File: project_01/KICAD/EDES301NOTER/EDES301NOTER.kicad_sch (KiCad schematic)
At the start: 39 parts, among them Q1 S8050, Q2 BSS84, Q3 BSS84, Q4 BSS84, Q5 BSS138, Q7 BSS138, SW1 SW_Reed, U1 POCKETBEAGLE, U3 TPS613222ADBVR

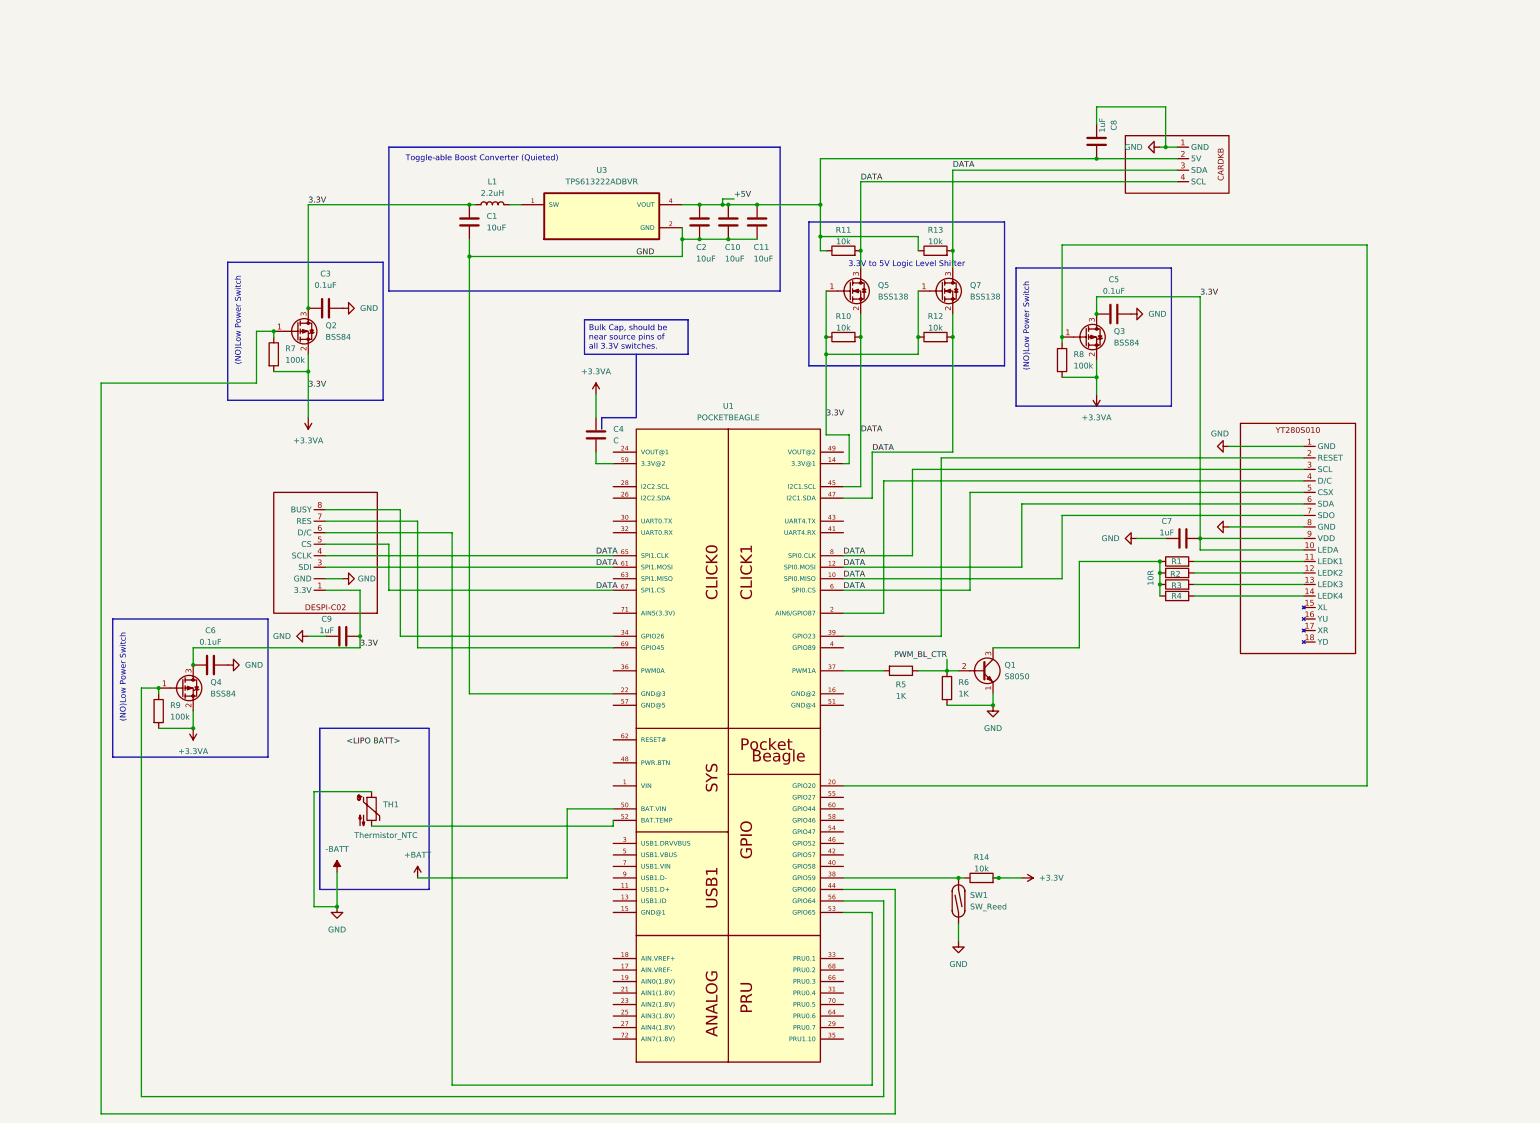
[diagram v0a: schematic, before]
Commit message: UpdateSchematicV1
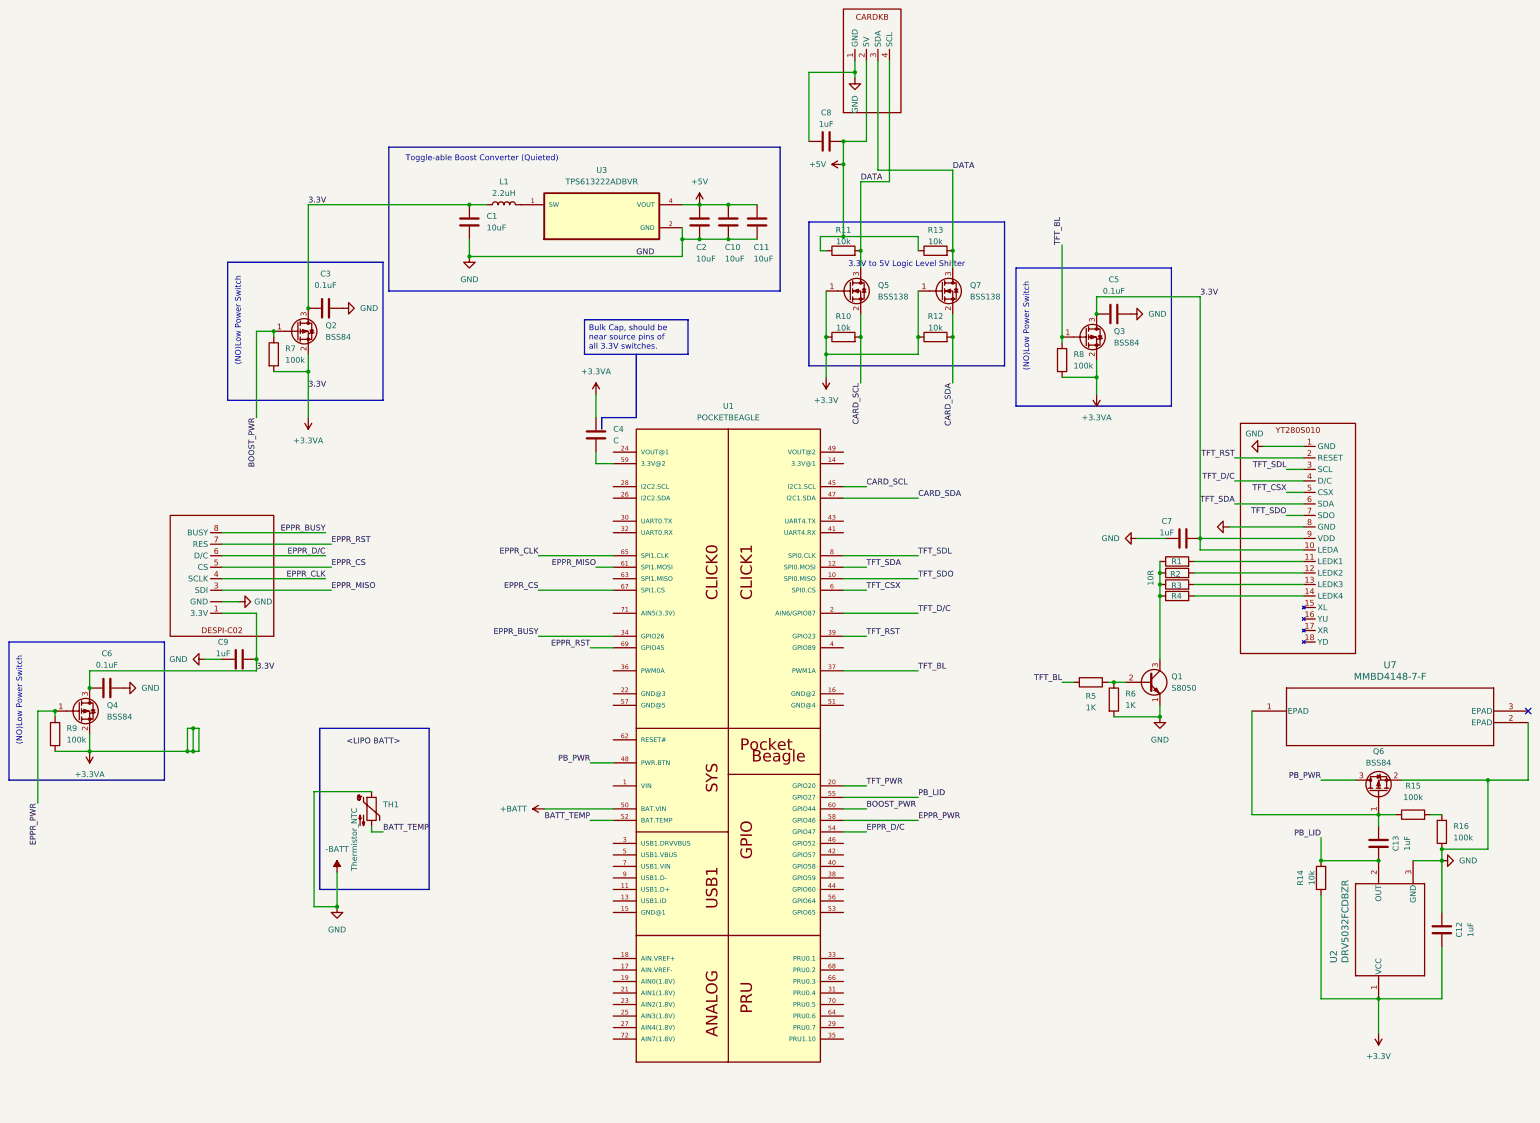
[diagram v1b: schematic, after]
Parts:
- removed SW1: SW_Reed, symbol Switch:SW_Reed
- added C12, C13: 1uF, Footprints:CAPC1608X90N, symbol Device:C
- added Q6: BSS84, Package_TO_SOT_SMD:SOT-23, symbol Transistor_FET:BSS84
- added R15, R16: 100k, Footprints:RESC1607X60N, symbol Device:R
- added U2: DRV5032FCDBZR, DBZ0003A-IPC_A, symbol DRV5032FCDBZR:DRV5032FCDBZR
- added U7: MMBD4148-7-F, SOT-23_DIO, symbol MMBD4148-7-F:MMBD4148-7-F
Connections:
- net +3.3V: now also Q5.1 (G), Q7.1 (G), R10.1, R12.1, R14.1, C12.1, U2.1 (VCC); no longer R14.2
- net +3.3VA: no longer Q5.1 (G), Q7.1 (G), R10.1, R12.1, U1.14 (3.3V@1)
- net -BATT: now also C12.2, Q6.2 (S), R16.1, U2.3 (GND), U7.2 (EPAD); no longer U1.22 (GND@3)
- net DATA: now also Q7.3 (D), R13.2, U4.3 (SDA); no longer Q5.2 (S), Q7.2 (S), R10.2, R12.2, U1.10 (SPI0.MISO), U1.12 (SPI0.MOSI), U1.45 (I2C1.SCL), U1.47 (I2C1.SDA), U1.6 (SPI0.CS), U1.61 (SPI1.MOSI), U1.65 (SPI1.CLK), U1.67 (SPI1.CS), U1.8 (SPI0.CLK), U5.3 (SCL), U5.5 (CSX), U5.6 (SDA), U5.7 (SDO), U6.3 (SDI), U6.4 (SCLK), U6.5 (CS)
- net at U1.38 (GPIO59): no longer R14.1
- net EPPR_PWR: now reaches Q4.1 (G), R9.1
- net EPPR_PWR: now also U1.58 (GPIO46); no longer U1.56 (GPIO64)
- net at U1.53 (GPIO65): no longer U6.6 (D/C)
- net EPPR_RST: now reaches U1.69 (GPIO45), U6.7 (RES)
- net EPPR_BUSY: now reaches U1.34 (GPIO26), U6.8 (BUSY)
- net TFT_BL: now reaches R5.2, U1.37 (PWM1A)
- net TFT_BL: now also Q3.1 (G), R8.1
- net BATT_TEMP: now reaches TH1.2, U1.52 (BAT.TEMP)
- net BOOST_PWR: now reaches Q2.1 (G), R7.1
- net BOOST_PWR: now also U1.60 (GPIO44); no longer U1.44 (GPIO60)
- net TFT_D/C: now reaches U1.2 (AIN6/GPIO87), U5.4 (D/C)
- net TFT_RST: now reaches U1.39 (GPIO23), U5.2 (RESET)
- net PB_PWR: now reaches U1.48 (PWR.BTN)
- net PB_PWR: now also Q6.3 (D)
- net EPPR_D/C: now reaches U1.54 (GPIO47)
- net EPPR_D/C: now also U6.6 (D/C)
- net PB_LID: now reaches U1.55 (GPIO27)
- net PB_LID: now also R14.2, C13.1, U2.2 (OUT)
- net PWM_BL_CTR: no longer names the net of Q1.2 (B), R5.1, R6.1
- new net: R15.2, R16.2
- new net: C13.2, Q6.1 (G), R15.1, U7.1 (EPAD)
- new net CARD_SCL: Q5.2 (S), R10.2, U1.45 (I2C1.SCL)
- new net CARD_SDA: Q7.2 (S), R12.2, U1.47 (I2C1.SDA)
- new net EPPR_CLK: U1.65 (SPI1.CLK), U6.4 (SCLK)
- new net EPPR_CS: U1.67 (SPI1.CS), U6.5 (CS)
- new net EPPR_MISO: U1.61 (SPI1.MOSI), U6.3 (SDI)
- new net TFT_CSX: U1.6 (SPI0.CS), U5.5 (CSX)
- new net TFT_PWR: U1.20 (GPIO20)
- new net TFT_SDA: U1.12 (SPI0.MOSI), U5.6 (SDA)
- new net TFT_SDL: U1.8 (SPI0.CLK), U5.3 (SCL)
- new net TFT_SDO: U1.10 (SPI0.MISO), U5.7 (SDO)
- no-connect marks 0 -> 1
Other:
- moved on the sheet: C6, C8, C9, L1, Q1, Q4, R5, R6, R9
